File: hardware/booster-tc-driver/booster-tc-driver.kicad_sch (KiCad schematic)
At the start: 144 parts, among them IC1 AD5160BRJZ5-RL7, IC2 AD5160BRJZ5-RL7, IC3 BD50FD0WHFP-TR, IC4 CAT4109V-GT2, IC5 L4940D2T12-TR, J1 62201021121, J10 3-647166-2, J2 EHT-105-01-S-D, J3 3-647166-2, J6 22-23-2021, J7 3-647166-2, J8 B4B-PH-SM4-TB, Q1 T2N7002AK, SW1 SW_SPDT, U1 STM32G474CBTx, U10 LT1963AxST-3.3, U2 AOZ1284PI, U3 CSTNE8M00G550000R0, U4 IF-D95T << must be T, U5 IF-E96E, U6 IF-D95T << must be T, U7 AOZ1284PI

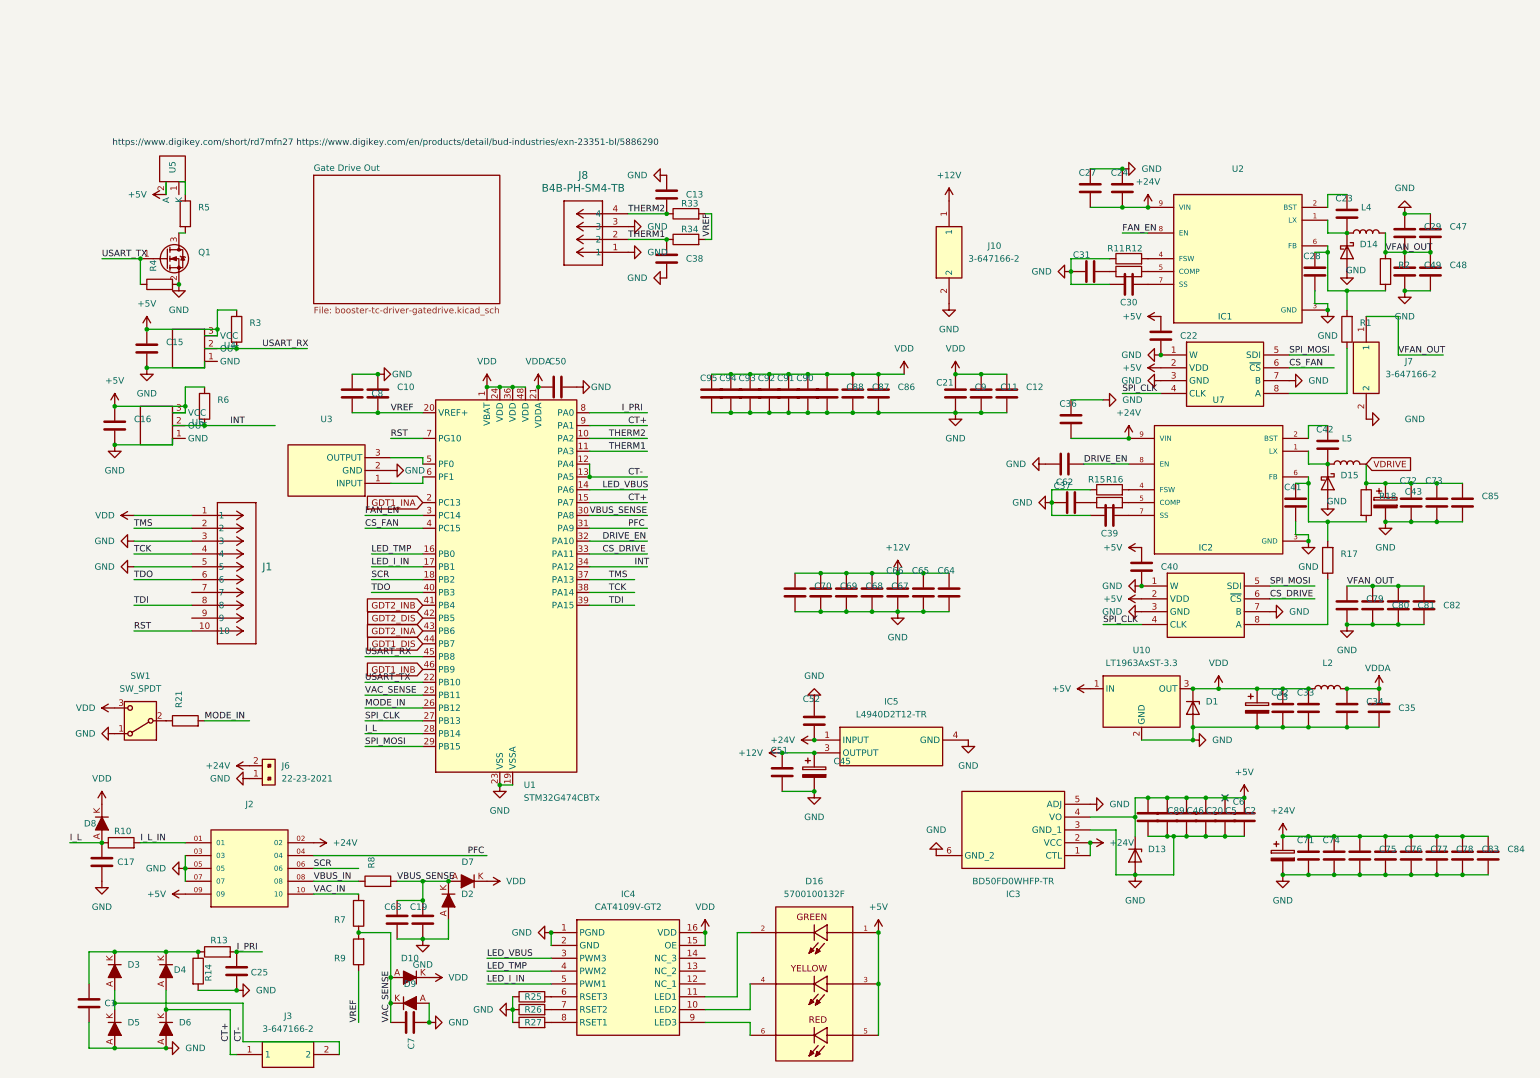
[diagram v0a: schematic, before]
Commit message: schematic cleanup
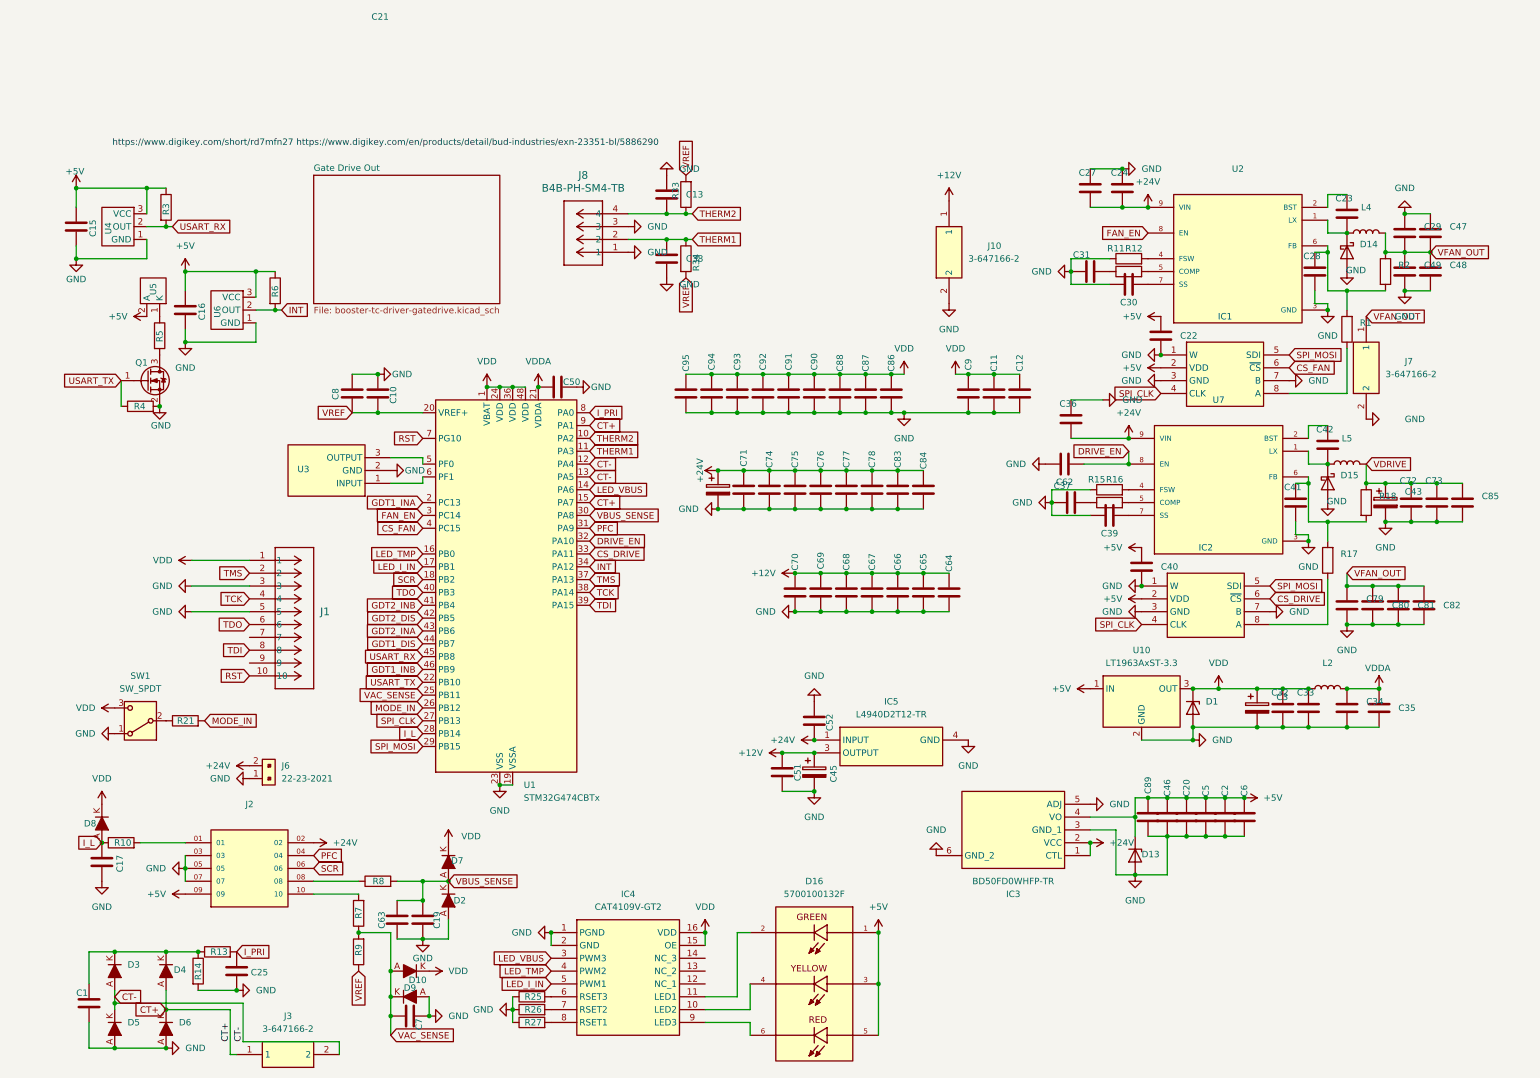
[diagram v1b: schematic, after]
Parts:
- L4, L5: value 22u 7443551221 -> 22u SRP7028A-220M; footprint Library:7443551221 -> Library:INDPM7366X300N
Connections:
- net I_L_IN: no longer names the net of J2.01, R10.2
- net VAC_IN: no longer names the net of J2.10, R7.2
- net VBUS_IN: no longer names the net of J2.08, R8.1
- no-connect marks 1 -> 0
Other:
- moved on the sheet: C11, C12, C15, C16, C21, C7, C71, C74, C75, C76, C77, C78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
